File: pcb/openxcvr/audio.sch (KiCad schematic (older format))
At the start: 28 parts, among them J1 Microphone, J2 Mic, J3 Speaker, J4 Headphone, U2 TPA711D, U3 MCP6002-xSN

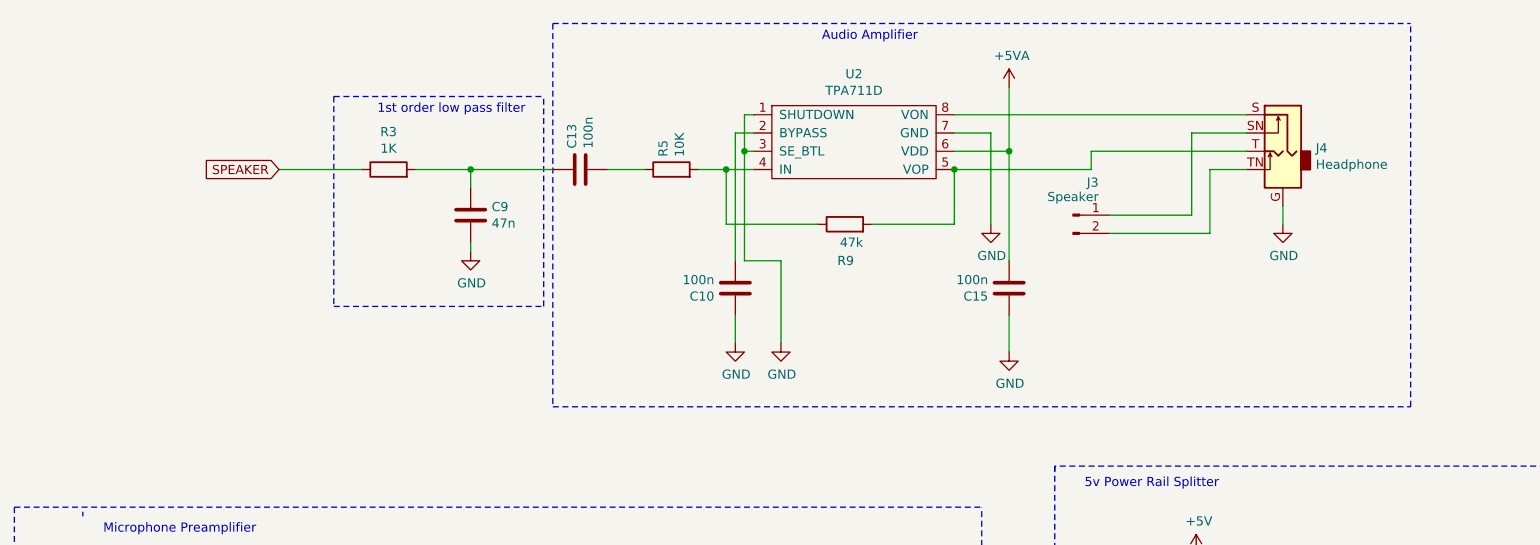
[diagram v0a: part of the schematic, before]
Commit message: PCB reviewed and updated
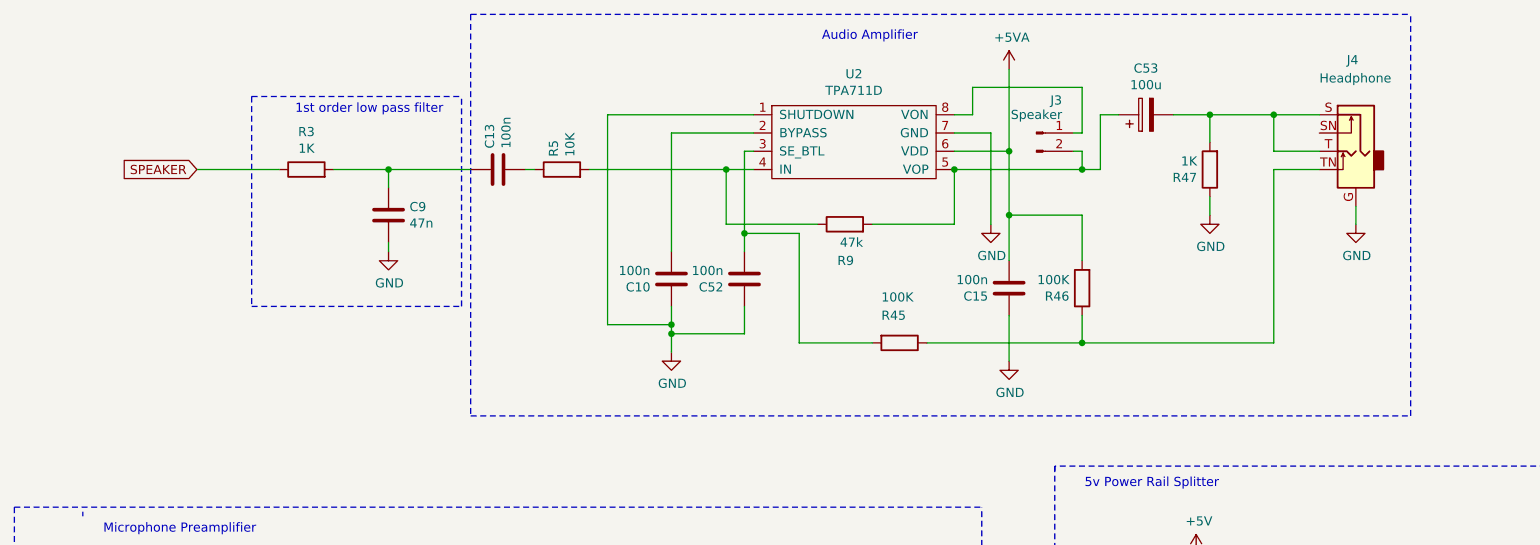
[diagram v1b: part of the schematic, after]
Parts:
- added C52: 100n, Capacitor_SMD:C_0805_2012Metric, symbol Device:C
- added C53: 100u, Capacitor_Tantalum_SMD:CP_EIA-7343-31_Kemet-D, symbol Device:CP
- added R45, R46: 100K, Resistor_SMD:R_0805_2012Metric, symbol Device:R
- added R47: 1K, Resistor_SMD:R_0805_2012Metric, symbol Device:R
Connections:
- wire segments 118 -> 141
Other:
- moved on the sheet: C10, C13, C9, J3, J4, R3, R5
